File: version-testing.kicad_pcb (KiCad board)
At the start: 2 copper layers, 52.5 x 24.1 mm, 0 parts

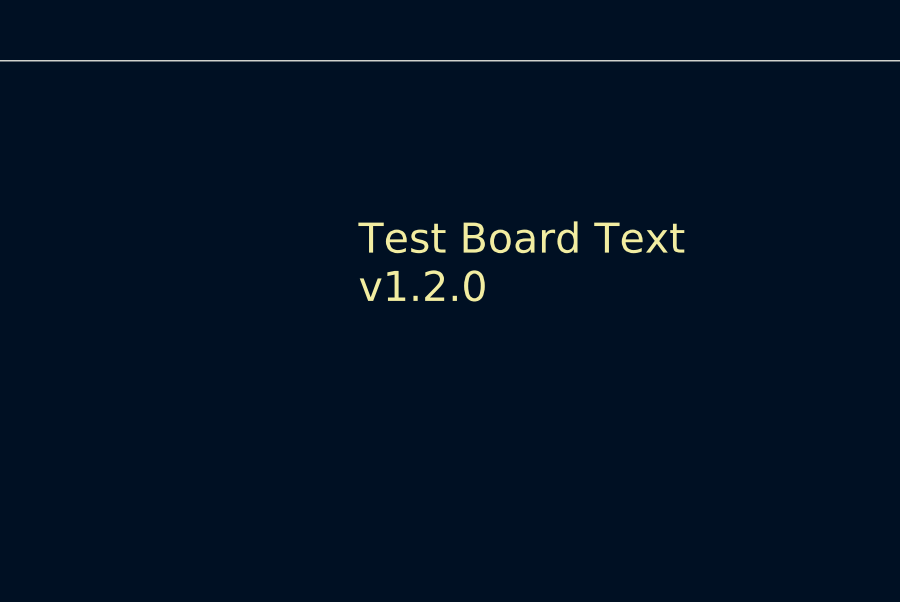
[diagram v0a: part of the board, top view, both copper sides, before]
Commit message: fix: version
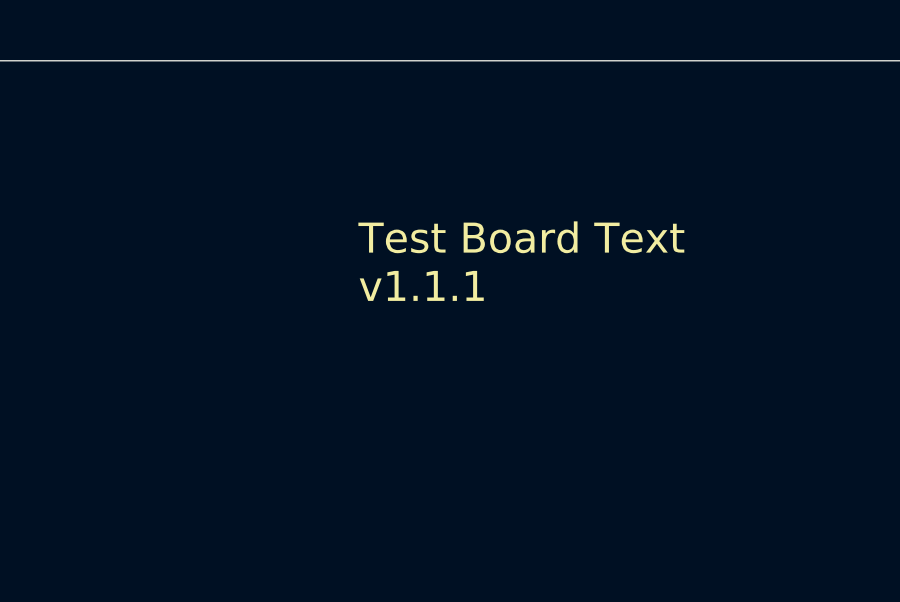
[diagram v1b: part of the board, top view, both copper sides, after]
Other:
- board text added: "Test Board Text v1.1.1"
- board text removed: "Test Board Text v1.2.0"
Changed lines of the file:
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@@
 		(layer "Edge.Cuts")
 	)
-	(gr_text "Test Board Text\nv1.2.0"
+	(gr_text "Test Board Text\nv1.1.1"
 		(at 84.963 33.528 0)
 		(layer "F.SilkS")
@@
 			(justify left bottom)
 		)
-		(render_cache "Test Board Text\nv1.2.0" 0
+		(render_cache "Test Board Text\nv1.1.1" 0
 			(polygon
 				(pts
@@
 			(polygon
 				(pts
-					(xy 87.744254 33.240763) (xy 88.212895 33.240763) (xy 88.212895 33.358) (xy 87.593312 33.358) (xy 87.593312 33.240763)
-					(xy 87.816672 33.003359) (xy 87.948502 32.858034) (xy 88.009433 32.777261) (xy 88.040704 32.723334)
-					(xy 88.058732 32.670866) (xy 88.064639 32.617883) (xy 88.05859 32.563164) (xy 88.041661 32.519437)
-					(xy 88.014386 32.484221) (xy 87.978178 32.458013) (xy 87.933136 32.441617) (xy 87.876756 32.435739)
-					(xy 87.814235 32.44111) (xy 87.746269 32.458026) (xy 87.677964 32.485128) (xy 87.601494 32.52562)
-					(xy 87.601494 32.384936) (xy 87.672139 32.355748) (xy 87.739796 32.335294) (xy 87.807829 32.322643)
-					(xy 87.874069 32.318502) (xy 87.948513 32.323978) (xy 88.012339 32.339511) (xy 88.067316 32.364268)
-					(xy 88.114831 32.398125) (xy 88.154709 32.440956) (xy 88.182864 32.489189) (xy 88.200076 32.54392)
-					(xy 88.206056 32.60677) (xy 88.198636 32.671573) (xy 88.175648 32.737989) (xy 88.138155 32.803436)
-					(xy 88.076913 32.882764) (xy 87.965904 33.005801)
+					(xy 87.673912 33.240763) (xy 87.888418 33.240763) (xy 87.888418 32.472131) (xy 87.631536 32.595473)
+					(xy 87.631536 32.463216) (xy 87.887014 32.341949) (xy 88.025011 32.341949) (xy 88.025011 33.240763)
+					(xy 88.23677 33.240763) (xy 88.23677 33.358) (xy 87.673912 33.358)
 				)
 			)
@@
 			(polygon
 				(pts
-					(xy 89.658353 32.328056) (xy 89.713589 32.344224) (xy 89.761844 32.370439) (xy 89.804269 32.407153)
-					(xy 89.841445 32.455705) (xy 89.875035 32.522523) (xy 89.901319 32.607767) (xy 89.91876 32.715404)
-					(xy 89.925159 32.849974) (xy 89.918761 32.984541) (xy 89.901321 33.09219) (xy 89.875037 33.177458)
-					(xy 89.841445 33.244304) (xy 89.804272 33.292832) (xy 89.761849 33.329529) (xy 89.713595 33.355732)
-					(xy 89.658356 33.371894) (xy 89.594516 33.377539) (xy 89.530697 33.371892) (xy 89.475512 33.355727)
-					(xy 89.427335 33.329523) (xy 89.385009 33.292829) (xy 89.347952 33.244304) (xy 89.314517 33.177481)
-					(xy 89.307739 33.1554) (xy 89.447665 33.1554) (xy 89.478445 33.207889) (xy 89.512714 33.241966)
-					(xy 89.550875 33.261519) (xy 89.594577 33.268118) (xy 89.639488 33.261816) (xy 89.677543 33.243473)
-					(xy 89.710523 33.212202) (xy 89.738985 33.164987) (xy 89.757575 33.114396) (xy 89.772567 33.047542)
-					(xy 89.78272 32.960792) (xy 89.78649 32.850096) (xy 89.782884 32.740094) (xy 89.772813 32.64652)
-					(xy 89.447665 33.1554) (xy 89.307739 33.1554) (xy 89.288346 33.092223) (xy 89.270977 32.984566)
-					(xy 89.264605 32.849974) (xy 89.264608 32.849913) (xy 89.403273 32.849913) (xy 89.40663 32.944583)
-					(xy 89.416279 33.030226) (xy 89.734589 32.522689) (xy 89.704741 32.481136) (xy 89.671967 32.453479)
-					(xy 89.635698 32.437318) (xy 89.594577 32.431831) (xy 89.549988 32.438117) (xy 89.512119 32.45644)
-					(xy 89.479209 32.487724) (xy 89.450718 32.535023) (xy 89.432152 32.585611) (xy 89.41718 32.652464)
-					(xy 89.407039 32.739215) (xy 89.403273 32.849913) (xy 89.264608 32.849913) (xy 89.270978 32.71538)
-					(xy 89.288348 32.607734) (xy 89.314519 32.522499) (xy 89.347952 32.455705) (xy 89.385012 32.407156)
-					(xy 89.42734 32.370444) (xy 89.475518 32.34423) (xy 89.530701 32.328059) (xy 89.594516 32.32241)
-				)
-			)
+					(xy 89.358211 33.240763) (xy 89.572717 33.240763) (xy 89.572717 32.472131) (xy 89.315834 32.595473)
+					(xy 89.315834 32.463216) (xy 89.571312 32.341949) (xy 89.70931 32.341949) (xy 89.70931 33.240763)
+					(xy 89.921068 33.240763) (xy 89.921068 33.358) (xy 89.358211 33.358)
+				)
+			)

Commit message: bump: version 1.1.1 → 1.1.2
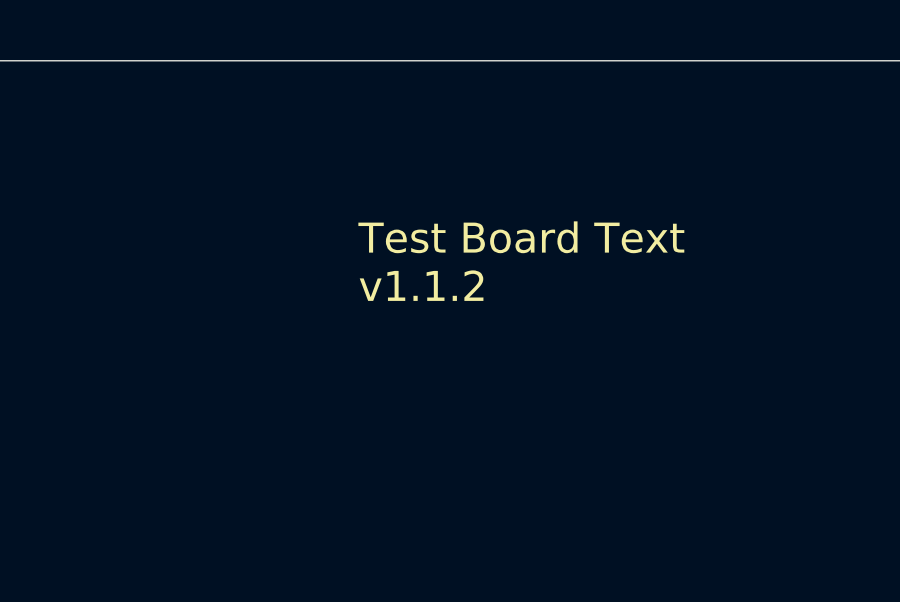
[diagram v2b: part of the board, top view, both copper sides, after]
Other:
- board text added: "Test Board Text v1.1.2"
- board text removed: "Test Board Text v1.1.1"
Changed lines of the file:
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@@
 		(layer "Edge.Cuts")
 	)
-	(gr_text "Test Board Text\nv1.1.1"
+	(gr_text "Test Board Text\nv1.1.2"
 		(at 84.963 33.528 0)
 		(layer "F.SilkS")
@@
 			(justify left bottom)
 		)
-		(render_cache "Test Board Text\nv1.1.1" 0
+		(render_cache "Test Board Text\nv1.1.2" 0
 			(polygon
 				(pts
@@
 			(polygon
 				(pts
-					(xy 89.358211 33.240763) (xy 89.572717 33.240763) (xy 89.572717 32.472131) (xy 89.315834 32.595473)
-					(xy 89.315834 32.463216) (xy 89.571312 32.341949) (xy 89.70931 32.341949) (xy 89.70931 33.240763)
-					(xy 89.921068 33.240763) (xy 89.921068 33.358) (xy 89.358211 33.358)
-				)
-			)
+					(xy 89.428553 33.240763) (xy 89.897193 33.240763) (xy 89.897193 33.358) (xy 89.27761 33.358) (xy 89.27761 33.240763)
+					(xy 89.500971 33.003359) (xy 89.632801 32.858034) (xy 89.693731 32.777261) (xy 89.725002 32.723334)
+					(xy 89.743031 32.670866) (xy 89.748938 32.617883) (xy 89.742888 32.563164) (xy 89.725959 32.519437)
+					(xy 89.698685 32.484221) (xy 89.662477 32.458013) (xy 89.617434 32.441617) (xy 89.561054 32.435739)
+					(xy 89.498533 32.44111) (xy 89.430568 32.458026) (xy 89.362263 32.485128) (xy 89.285793 32.52562)
+					(xy 89.285793 32.384936) (xy 89.356437 32.355748) (xy 89.424095 32.335294) (xy 89.492128 32.322643)
+					(xy 89.558368 32.318502) (xy 89.632812 32.323978) (xy 89.696638 32.339511) (xy 89.751614 32.364268)
+					(xy 89.79913 32.398125) (xy 89.839007 32.440956) (xy 89.867163 32.489189) (xy 89.884375 32.54392)
+					(xy 89.890355 32.60677) (xy 89.882935 32.671573) (xy 89.859946 32.737989) (xy 89.822453 32.803436)
+					(xy 89.761211 32.882764) (xy 89.650203 33.005801)
+				)
+			)

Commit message: bump: version 1.1.2 → 1.1.3
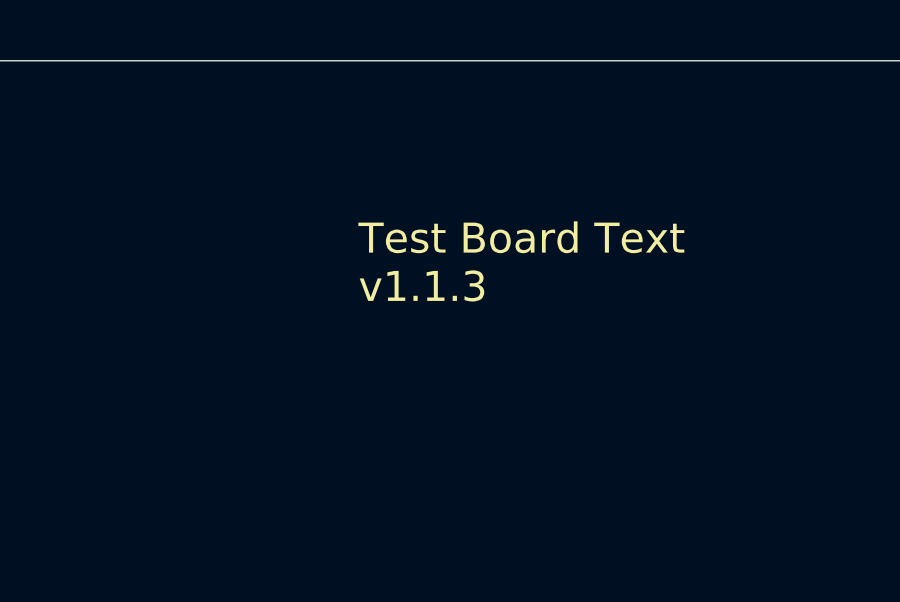
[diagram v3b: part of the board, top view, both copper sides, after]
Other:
- board text added: "Test Board Text v1.1.3"
- board text removed: "Test Board Text v1.1.2"
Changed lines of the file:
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@@
 		(layer "Edge.Cuts")
 	)
-	(gr_text "Test Board Text\nv1.1.2"
+	(gr_text "Test Board Text\nv1.1.3"
 		(at 84.963 33.528 0)
 		(layer "F.SilkS")
@@
 			(justify left bottom)
 		)
-		(render_cache "Test Board Text\nv1.1.2" 0
+		(render_cache "Test Board Text\nv1.1.3" 0
 			(polygon
 				(pts
@@
 			(polygon
 				(pts
-					(xy 89.428553 33.240763) (xy 89.897193 33.240763) (xy 89.897193 33.358) (xy 89.27761 33.358) (xy 89.27761 33.240763)
-					(xy 89.500971 33.003359) (xy 89.632801 32.858034) (xy 89.693731 32.777261) (xy 89.725002 32.723334)
-					(xy 89.743031 32.670866) (xy 89.748938 32.617883) (xy 89.742888 32.563164) (xy 89.725959 32.519437)
-					(xy 89.698685 32.484221) (xy 89.662477 32.458013) (xy 89.617434 32.441617) (xy 89.561054 32.435739)
-					(xy 89.498533 32.44111) (xy 89.430568 32.458026) (xy 89.362263 32.485128) (xy 89.285793 32.52562)
-					(xy 89.285793 32.384936) (xy 89.356437 32.355748) (xy 89.424095 32.335294) (xy 89.492128 32.322643)
-					(xy 89.558368 32.318502) (xy 89.632812 32.323978) (xy 89.696638 32.339511) (xy 89.751614 32.364268)
-					(xy 89.79913 32.398125) (xy 89.839007 32.440956) (xy 89.867163 32.489189) (xy 89.884375 32.54392)
-					(xy 89.890355 32.60677) (xy 89.882935 32.671573) (xy 89.859946 32.737989) (xy 89.822453 32.803436)
-					(xy 89.761211 32.882764) (xy 89.650203 33.005801)
-				)
-			)
+					(xy 89.703875 32.812178) (xy 89.767542 32.835474) (xy 89.818025 32.86704) (xy 89.857504 32.906761)
+					(xy 89.886552 32.954539) (xy 89.904501 33.010425) (xy 89.91081 33.076449) (xy 89.904454 33.145275)
+					(xy 89.886362 33.203792) (xy 89.857127 33.25401) (xy 89.816166 33.297305) (xy 89.767145 33.330884)
+					(xy 89.708475 33.355883) (xy 89.638274 33.371838) (xy 89.554215 33.377539) (xy 89.483657 33.374315)
+					(xy 89.410784 33.364472) (xy 89.338418 33.348545) (xy 89.267352 33.326736) (xy 89.267352 33.18996)
+					(xy 89.337474 33.221307) (xy 89.404617 33.2429) (xy 89.472444 33.255996) (xy 89.539256 33.260302)
+					(xy 89.613261 33.253844) (xy 89.670035 33.23629) (xy 89.713401 33.209256) (xy 89.739429 33.181705)
+					(xy 89.758237 33.148806) (xy 89.770029 33.109474) (xy 89.774217 33.06216) (xy 89.767125 33.005976)
+					(xy 89.746906 32.959921) (xy 89.713401 32.921599) (xy 89.670112 32.893602) (xy 89.616192 32.875892)
+					(xy 89.548781 32.869514) (xy 89.443573 32.869514) (xy 89.443573 32.756185) (xy 89.548781 32.756185)
+					(xy 89.61085 32.750953) (xy 89.659282 32.73665) (xy 89.696975 32.714542) (xy 89.726374 32.683414)
+					(xy 89.744062 32.645409) (xy 89.750281 32.598343) (xy 89.744322 32.548222) (xy 89.727689 32.508869)
+					(xy 89.700761 32.477748) (xy 89.665397 32.455451) (xy 89.619386 32.441029) (xy 89.559711 32.435739)
+					(xy 89.498544 32.439085) (xy 89.433987 32.449416) (xy 89.368761 32.466149) (xy 89.298066 32.490449)
+					(xy 89.298066 32.361489) (xy 89.445283 32.329249) (xy 89.508206 32.320999) (xy 89.559711 32.318502)
+					(xy 89.634126 32.32372) (xy 89.697459 32.338457) (xy 89.751528 32.361799) (xy 89.797787 32.393484)
+					(xy 89.83679 32.434033) (xy 89.864285 32.479889) (xy 89.881091 32.532124) (xy 89.886935 32.592359)
+					(xy 89.88143 32.646836) (xy 89.865712 32.69308) (xy 89.840102 32.732799) (xy 89.805652 32.765458)
+					(xy 89.760954 32.792014)
+				)
+			)

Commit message: bump: version 1.1.3 → 1.2.0
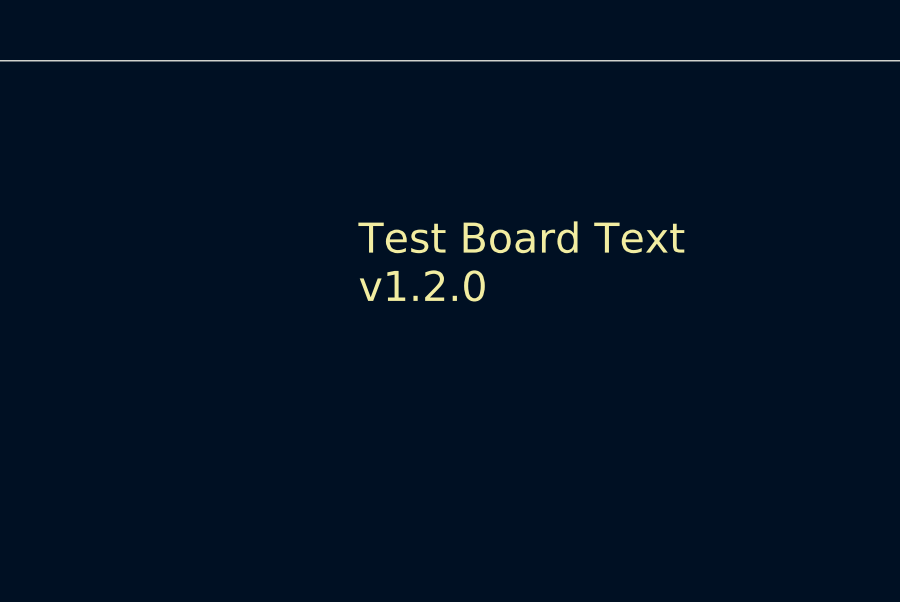
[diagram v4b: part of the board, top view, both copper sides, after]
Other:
- board text added: "Test Board Text v1.2.0"
- board text removed: "Test Board Text v1.1.3"
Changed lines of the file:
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@@
 		(layer "Edge.Cuts")
 	)
-	(gr_text "Test Board Text\nv1.1.3"
+	(gr_text "Test Board Text\nv1.2.0"
 		(at 84.963 33.528 0)
 		(layer "F.SilkS")
@@
 			(justify left bottom)
 		)
-		(render_cache "Test Board Text\nv1.1.3" 0
+		(render_cache "Test Board Text\nv1.2.0" 0
 			(polygon
 				(pts
@@
 			(polygon
 				(pts
-					(xy 87.673912 33.240763) (xy 87.888418 33.240763) (xy 87.888418 32.472131) (xy 87.631536 32.595473)
-					(xy 87.631536 32.463216) (xy 87.887014 32.341949) (xy 88.025011 32.341949) (xy 88.025011 33.240763)
-					(xy 88.23677 33.240763) (xy 88.23677 33.358) (xy 87.673912 33.358)
+					(xy 87.744254 33.240763) (xy 88.212895 33.240763) (xy 88.212895 33.358) (xy 87.593312 33.358) (xy 87.593312 33.240763)
+					(xy 87.816672 33.003359) (xy 87.948502 32.858034) (xy 88.009433 32.777261) (xy 88.040704 32.723334)
+					(xy 88.058732 32.670866) (xy 88.064639 32.617883) (xy 88.05859 32.563164) (xy 88.041661 32.519437)
+					(xy 88.014386 32.484221) (xy 87.978178 32.458013) (xy 87.933136 32.441617) (xy 87.876756 32.435739)
+					(xy 87.814235 32.44111) (xy 87.746269 32.458026) (xy 87.677964 32.485128) (xy 87.601494 32.52562)
+					(xy 87.601494 32.384936) (xy 87.672139 32.355748) (xy 87.739796 32.335294) (xy 87.807829 32.322643)
+					(xy 87.874069 32.318502) (xy 87.948513 32.323978) (xy 88.012339 32.339511) (xy 88.067316 32.364268)
+					(xy 88.114831 32.398125) (xy 88.154709 32.440956) (xy 88.182864 32.489189) (xy 88.200076 32.54392)
+					(xy 88.206056 32.60677) (xy 88.198636 32.671573) (xy 88.175648 32.737989) (xy 88.138155 32.803436)
+					(xy 88.076913 32.882764) (xy 87.965904 33.005801)
 				)
 			)
@@
 			(polygon
 				(pts
-					(xy 89.703875 32.812178) (xy 89.767542 32.835474) (xy 89.818025 32.86704) (xy 89.857504 32.906761)
-					(xy 89.886552 32.954539) (xy 89.904501 33.010425) (xy 89.91081 33.076449) (xy 89.904454 33.145275)
-					(xy 89.886362 33.203792) (xy 89.857127 33.25401) (xy 89.816166 33.297305) (xy 89.767145 33.330884)
-					(xy 89.708475 33.355883) (xy 89.638274 33.371838) (xy 89.554215 33.377539) (xy 89.483657 33.374315)
-					(xy 89.410784 33.364472) (xy 89.338418 33.348545) (xy 89.267352 33.326736) (xy 89.267352 33.18996)
-					(xy 89.337474 33.221307) (xy 89.404617 33.2429) (xy 89.472444 33.255996) (xy 89.539256 33.260302)
-					(xy 89.613261 33.253844) (xy 89.670035 33.23629) (xy 89.713401 33.209256) (xy 89.739429 33.181705)
-					(xy 89.758237 33.148806) (xy 89.770029 33.109474) (xy 89.774217 33.06216) (xy 89.767125 33.005976)
-					(xy 89.746906 32.959921) (xy 89.713401 32.921599) (xy 89.670112 32.893602) (xy 89.616192 32.875892)
-					(xy 89.548781 32.869514) (xy 89.443573 32.869514) (xy 89.443573 32.756185) (xy 89.548781 32.756185)
-					(xy 89.61085 32.750953) (xy 89.659282 32.73665) (xy 89.696975 32.714542) (xy 89.726374 32.683414)
-					(xy 89.744062 32.645409) (xy 89.750281 32.598343) (xy 89.744322 32.548222) (xy 89.727689 32.508869)
-					(xy 89.700761 32.477748) (xy 89.665397 32.455451) (xy 89.619386 32.441029) (xy 89.559711 32.435739)
-					(xy 89.498544 32.439085) (xy 89.433987 32.449416) (xy 89.368761 32.466149) (xy 89.298066 32.490449)
-					(xy 89.298066 32.361489) (xy 89.445283 32.329249) (xy 89.508206 32.320999) (xy 89.559711 32.318502)
-					(xy 89.634126 32.32372) (xy 89.697459 32.338457) (xy 89.751528 32.361799) (xy 89.797787 32.393484)
-					(xy 89.83679 32.434033) (xy 89.864285 32.479889) (xy 89.881091 32.532124) (xy 89.886935 32.592359)
-					(xy 89.88143 32.646836) (xy 89.865712 32.69308) (xy 89.840102 32.732799) (xy 89.805652 32.765458)
-					(xy 89.760954 32.792014)
-				)
-			)
+					(xy 89.658353 32.328056) (xy 89.713589 32.344224) (xy 89.761844 32.370439) (xy 89.804269 32.407153)
+					(xy 89.841445 32.455705) (xy 89.875035 32.522523) (xy 89.901319 32.607767) (xy 89.91876 32.715404)
+					(xy 89.925159 32.849974) (xy 89.918761 32.984541) (xy 89.901321 33.09219) (xy 89.875037 33.177458)
+					(xy 89.841445 33.244304) (xy 89.804272 33.292832) (xy 89.761849 33.329529) (xy 89.713595 33.355732)
+					(xy 89.658356 33.371894) (xy 89.594516 33.377539) (xy 89.530697 33.371892) (xy 89.475512 33.355727)
+					(xy 89.427335 33.329523) (xy 89.385009 33.292829) (xy 89.347952 33.244304) (xy 89.314517 33.177481)
+					(xy 89.307739 33.1554) (xy 89.447665 33.1554) (xy 89.478445 33.207889) (xy 89.512714 33.241966)
+					(xy 89.550875 33.261519) (xy 89.594577 33.268118) (xy 89.639488 33.261816) (xy 89.677543 33.243473)
+					(xy 89.710523 33.212202) (xy 89.738985 33.164987) (xy 89.757575 33.114396) (xy 89.772567 33.047542)
+					(xy 89.78272 32.960792) (xy 89.78649 32.850096) (xy 89.782884 32.740094) (xy 89.772813 32.64652)
+					(xy 89.447665 33.1554) (xy 89.307739 33.1554) (xy 89.288346 33.092223) (xy 89.270977 32.984566)
+					(xy 89.264605 32.849974) (xy 89.264608 32.849913) (xy 89.403273 32.849913) (xy 89.40663 32.944583)
+					(xy 89.416279 33.030226) (xy 89.734589 32.522689) (xy 89.704741 32.481136) (xy 89.671967 32.453479)
+					(xy 89.635698 32.437318) (xy 89.594577 32.431831) (xy 89.549988 32.438117) (xy 89.512119 32.45644)
+					(xy 89.479209 32.487724) (xy 89.450718 32.535023) (xy 89.432152 32.585611) (xy 89.41718 32.652464)
+					(xy 89.407039 32.739215) (xy 89.403273 32.849913) (xy 89.264608 32.849913) (xy 89.270978 32.71538)
+					(xy 89.288348 32.607734) (xy 89.314519 32.522499) (xy 89.347952 32.455705) (xy 89.385012 32.407156)
+					(xy 89.42734 32.370444) (xy 89.475518 32.34423) (xy 89.530701 32.328059) (xy 89.594516 32.32241)
+				)
+			)
